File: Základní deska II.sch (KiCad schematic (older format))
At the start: 2 parts, among them U1 ESP32-WROOM-32

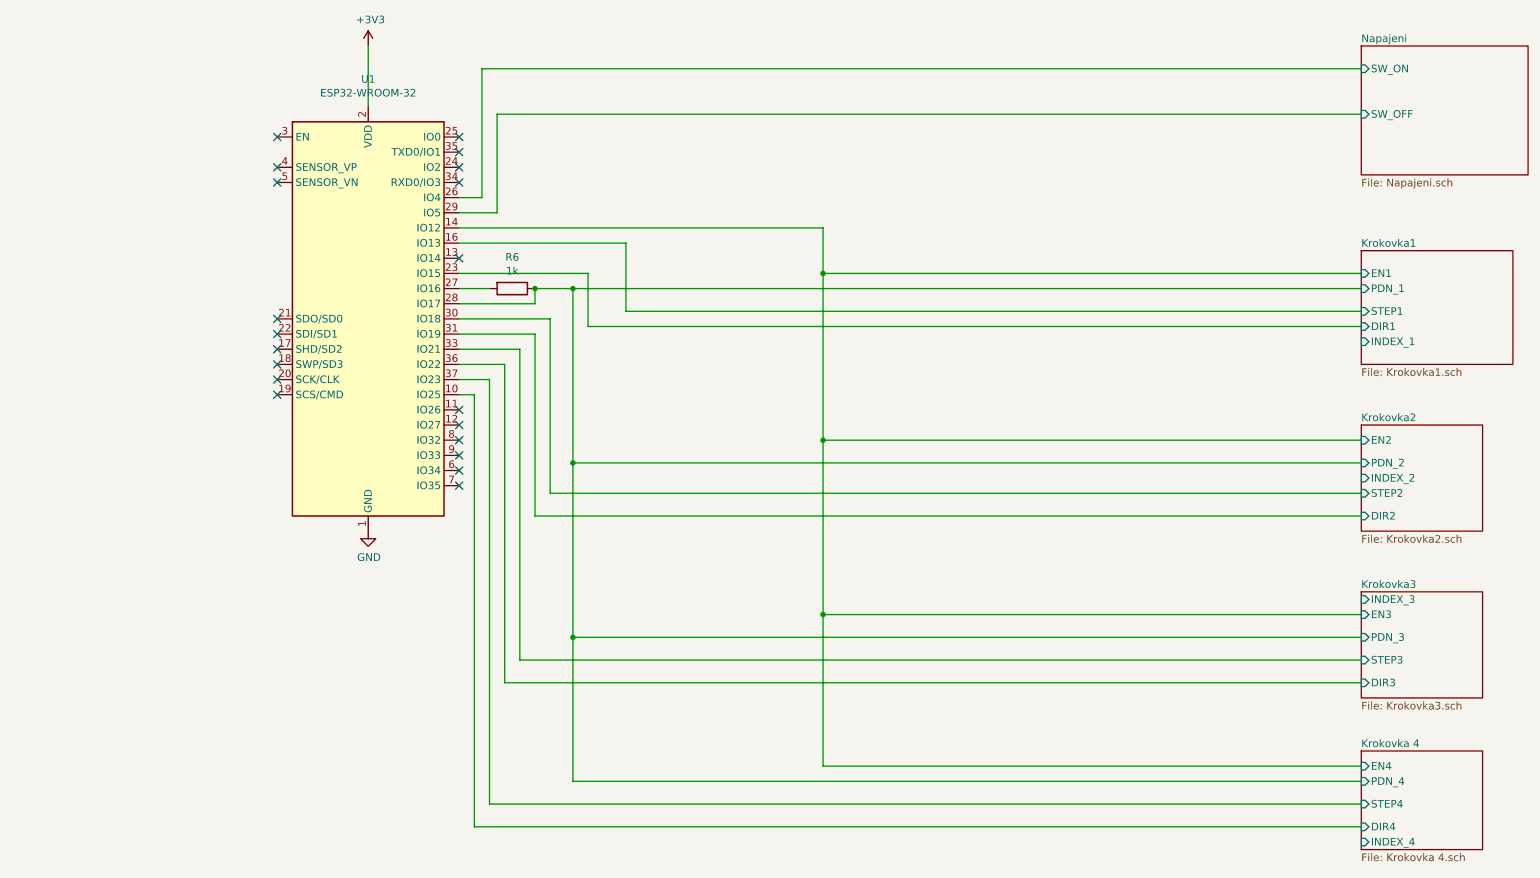
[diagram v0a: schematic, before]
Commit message: Deska 0.5
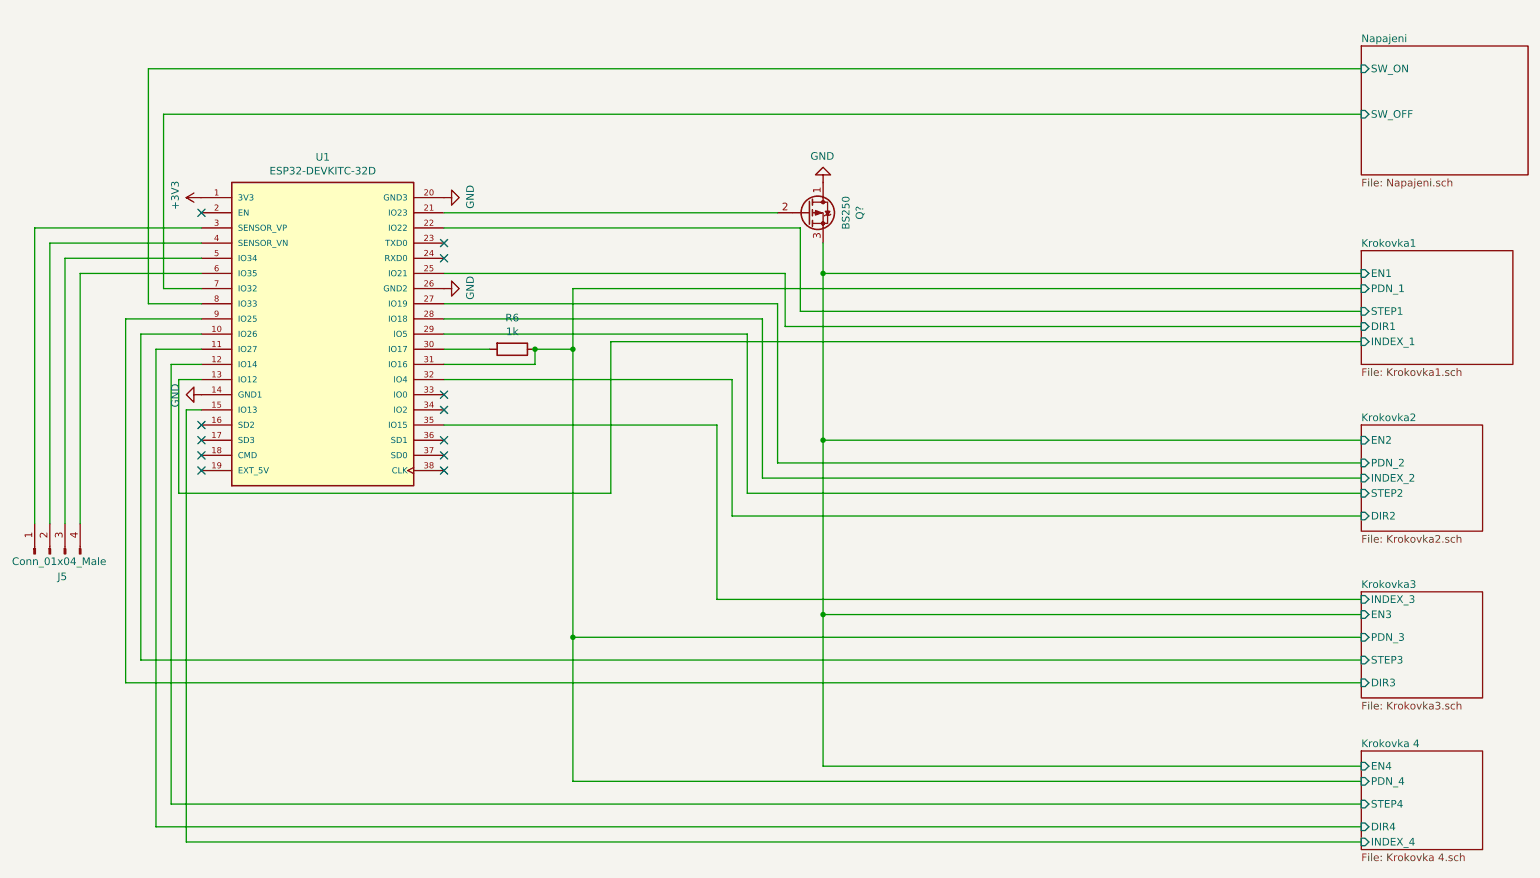
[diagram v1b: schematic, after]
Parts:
- removed U1: ESP32-WROOM-32, RF_Module:ESP32-WROOM-32, symbol RF_Module:ESP32-WROOM-32
- added J5: Conn_01x04_Male, symbol Connector:Conn_01x04_Male
- added Q?: BS250, Package_TO_SOT_THT:TO-92_Inline, symbol Transistor_FET:BS250
- added U1: ESP32-DEVKITC-32D, MODULE_ESP32-DEVKITC-32D, symbol ESP32-DEVKITC-32D:ESP32-DEVKITC-32D
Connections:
- net +3V3: now also U1.1 (3V3)
- net GND: now also Q?.1 (D), U1.14 (GND1), U1.20 (GND3), U1.26 (GND2)
- net Krokovka 4/DIR4: now also U1.11 (IO27)
- net Krokovka 4/EN4: now also Q?.3 (S)
- net Krokovka 4/INDEX_4: now also U1.15 (IO13)
- net Krokovka 4/PDN_4: now also U1.31 (IO16)
- net Krokovka 4/STEP4: now also U1.12 (IO14)
- net Krokovka1/DIR1: now also U1.25 (IO21)
- net Krokovka1/INDEX_1: now also U1.13 (IO12)
- net Krokovka1/STEP1: now also U1.22 (IO22)
- net Krokovka2/DIR2: now also U1.32 (IO4)
- net Krokovka2/INDEX_2: now also U1.28 (IO18)
- net Krokovka2/STEP2: now also U1.29 (IO5)
- net Krokovka3/DIR3: now also U1.9 (IO25)
- net Krokovka3/INDEX_3: now also U1.35 (IO15)
- net Krokovka3/STEP3: now also U1.10 (IO26)
- net Napajeni/SW_OFF: now also U1.7 (IO32)
- net Napajeni/SW_ON: now also U1.8 (IO33)
- net at R6.2: now also U1.30 (IO17)
- new net: Q?.2 (G), U1.21 (IO23)
- new net: J5.1 (Pin_1), U1.3 (SENSOR_VP)
- new net: J5.2 (Pin_2), U1.4 (SENSOR_VN)
- new net: J5.3 (Pin_3), U1.5 (IO34)
- new net: J5.4 (Pin_4), U1.6 (IO35)
- new net Krokovka2/PDN_2: U1.27 (IO19)
- no-connect marks 20 -> 12
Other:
- moved on the sheet: R6
